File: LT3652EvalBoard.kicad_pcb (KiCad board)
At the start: 2 copper layers, 49.8 x 49.8 mm, 45 parts, among them U1 LT3652

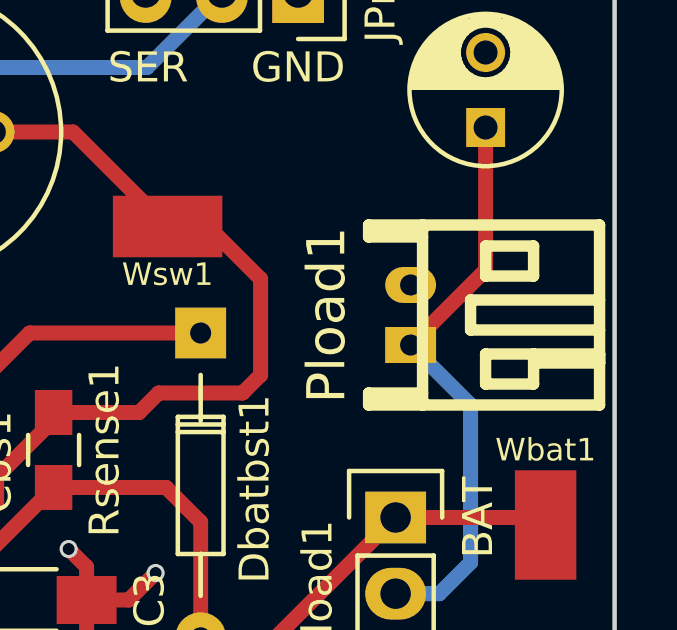
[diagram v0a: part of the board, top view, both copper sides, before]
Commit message: Minor alignment fix
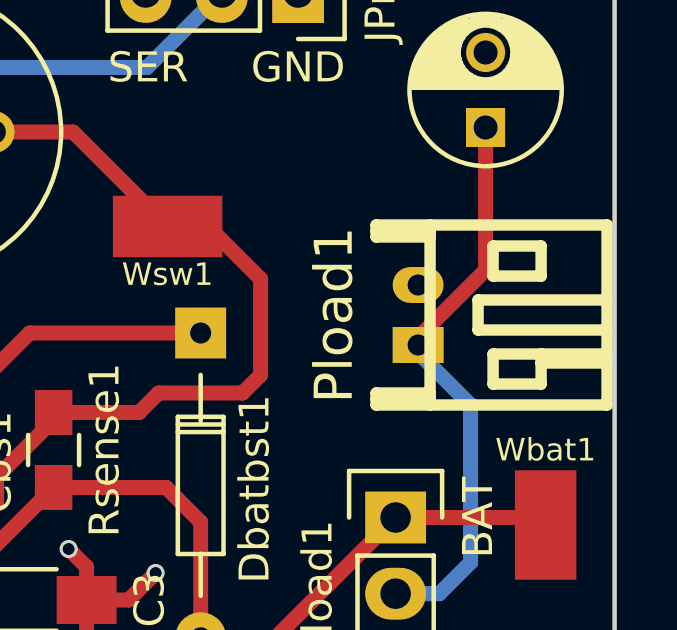
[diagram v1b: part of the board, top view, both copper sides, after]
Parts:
- moved Pload1 0.25 mm to (153.3, 85.0)
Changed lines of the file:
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@@
     (links 70)
     (no_connects 0)
-    (area 109.990999 65.274999 159.941001 115.225001)
+    (area 109.676715 62.92484 162.63554 117.28582)
     (thickness 1.6)
     (drawings 22)
@@
   )
   (setup
-    (last_trace_width 0.5)
+    (last_trace_width 0.25)
     (user_trace_width 0.3)
     (user_trace_width 0.4)
@@
   )
   (module w_conn_jst-ph:s2b-ph-kl (layer F.Cu)
-    (at 153.066 84.95 90)
+    (at 153.316 84.95 90)
     (descr "JST PH series connector, S2B-PH-KL")
     (fp_text reference Pload1 (at 0 -2.79908 90) (layer F.SilkS)
